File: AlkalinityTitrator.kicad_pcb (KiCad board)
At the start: 2 copper layers, 88.5 x 86.1 mm, 45 parts, among them J1 Conn_01x16, J10 Screw_Terminal_01x02, J12 V_OFFSET, J14 Conn_01x02, J2 Raspberry_Pi_2_3, J3 Conn_01x08, J4 Screw_Terminal_01x04_titrator, J5 RF_Shield_Two_Pieces, J7 SJ-43515TS, J8 Screw_Terminal_01x03, J9 SJ-43515TS, Q1 PN2222A, U1 ADS1115_BO, U2 A4988_BO, U3 MAX31865_BO, U4 MAX31865_BO, U5 LT1634, U6 LMC662, U7 LMC662, U8 L7805

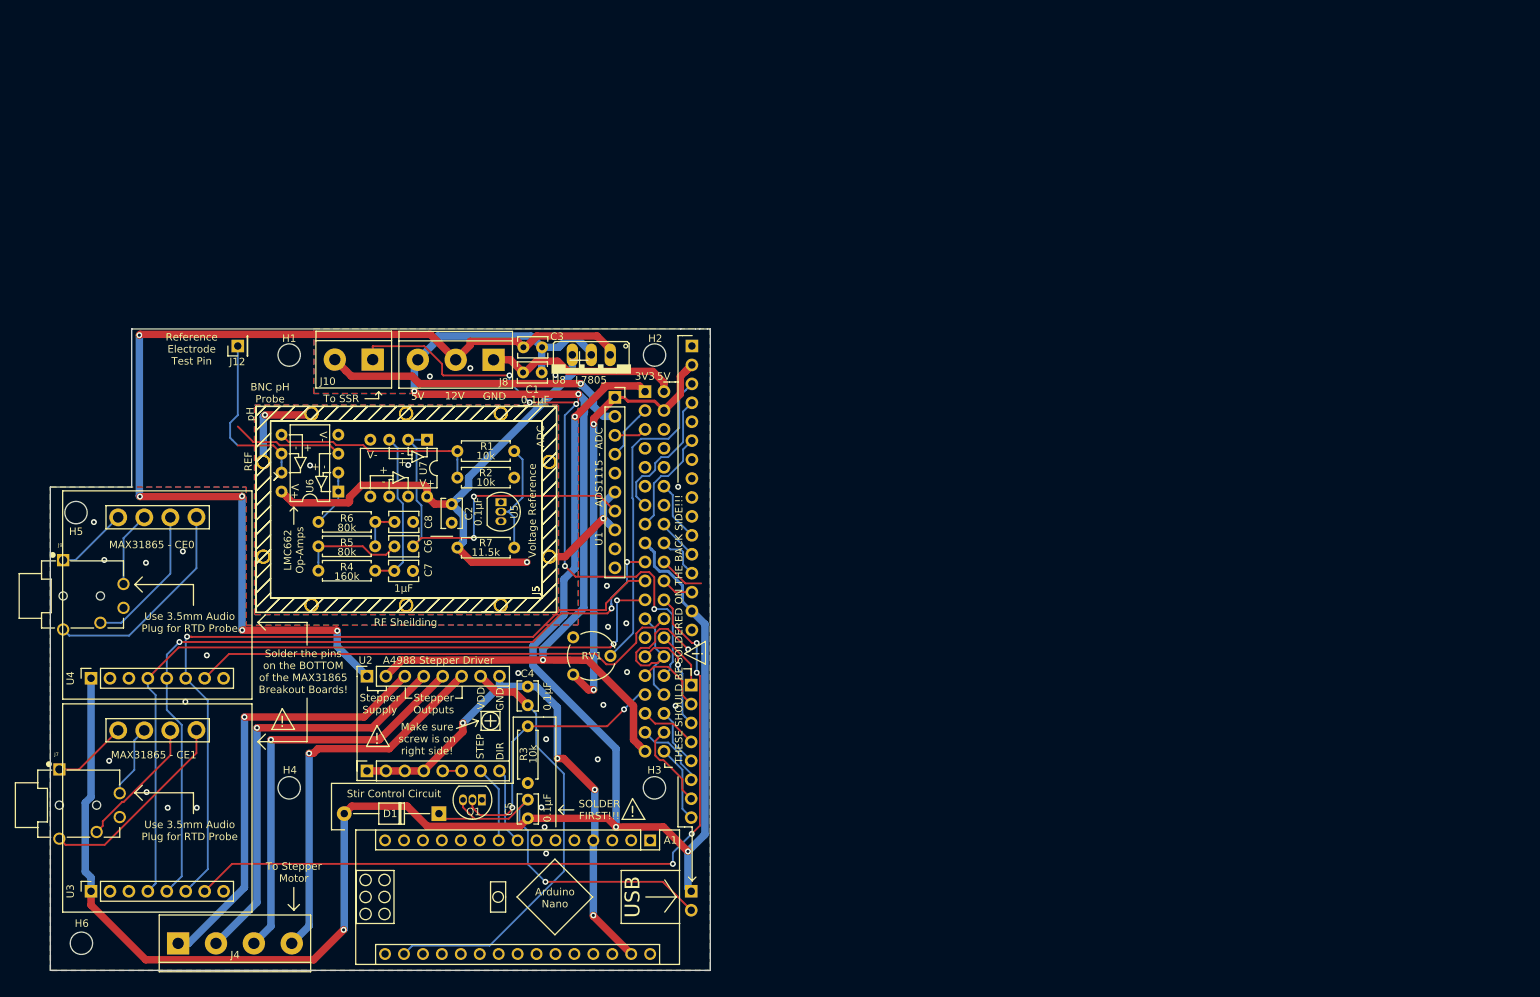
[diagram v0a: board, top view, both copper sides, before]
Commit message: rcb rev 3 start
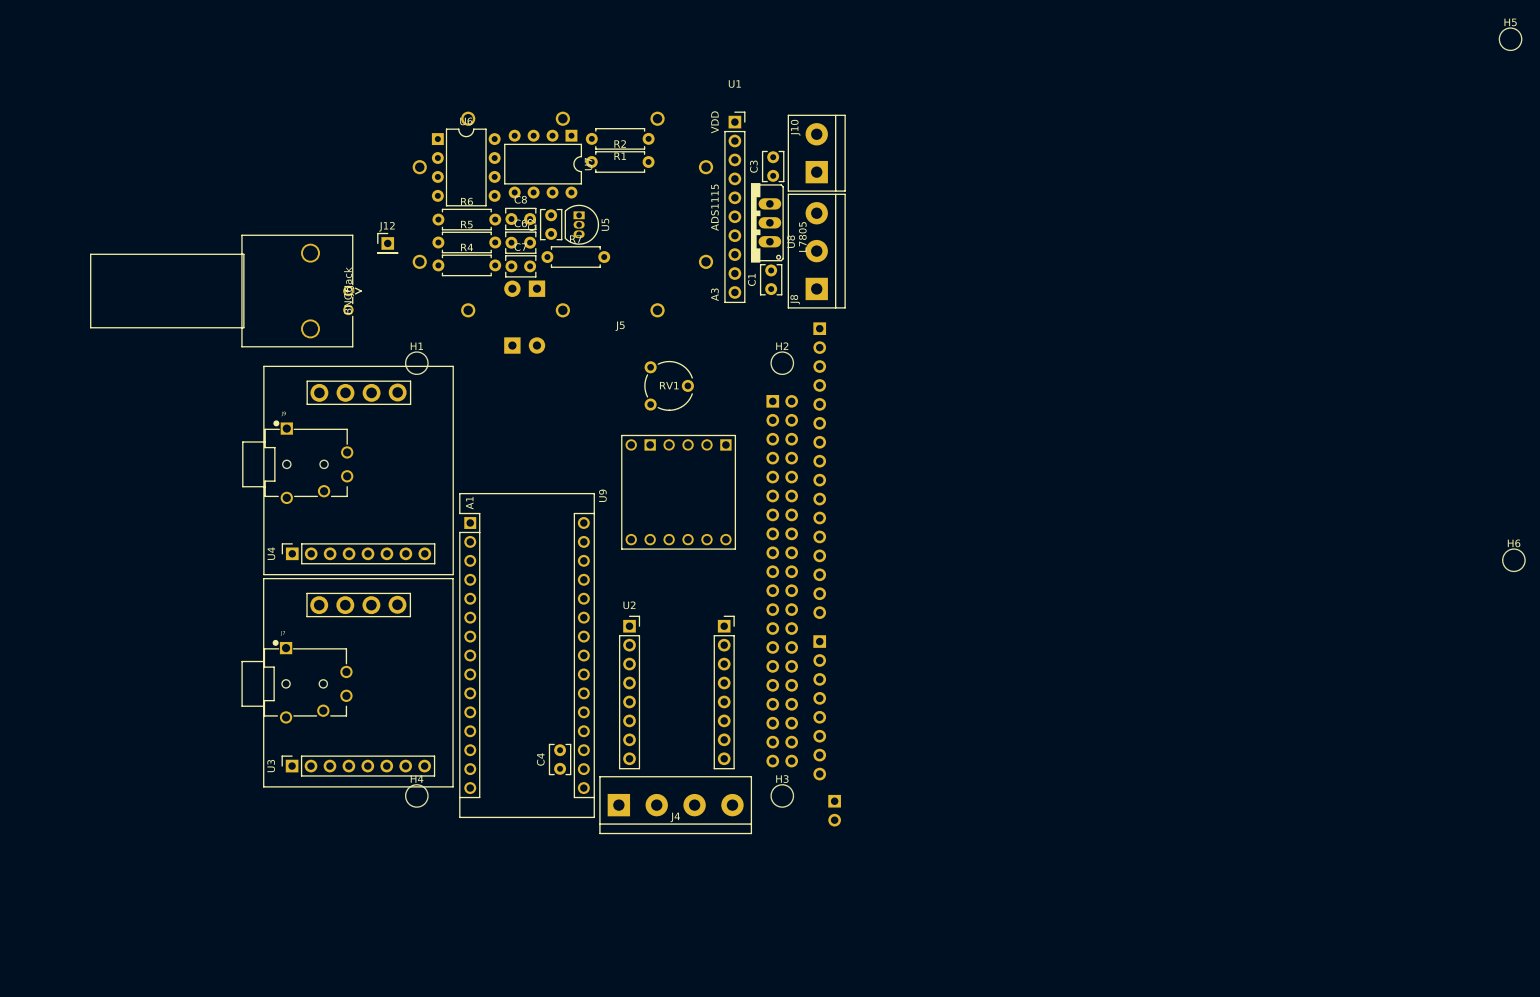
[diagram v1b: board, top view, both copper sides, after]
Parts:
- removed C5: 0.1uF, Capacitor_THT:C_Disc_D3.8mm_W2.6mm_P2.50mm
- removed the J5 at (148.2, 81.7) (x2)
- removed Q1: PN2222A, Package_TO_SOT_THT:TO-92_Inline
- removed R3: 10k, Resistor_THT:R_Axial_DIN0207_L6.3mm_D2.5mm_P7.62mm_Horizontal
- added D2: 1N5817-TP, Diode_THT:D_DO-41_SOD81_P7.62mm_Horizontal, B.Cu at (162.4, 58.9)
- added J5: RF_Shield_Two_Pieces, Titrator_Footprints:44-CBSA-1.0X1.5X0.4, F.Cu at (188.4, 54.1)
- added J6: BNC_Jack, Titrator_Footprints:BNC_Jack, F.Cu at (140.4, 51.5)
- added U9: BD65496MUV_BO, Titrator_Footprints:BD65496MUV_BO_Footprint, F.Cu at (174.8, 78.4)
- A1: footprint Module:Arduino_Nano -> Titrator_Footprints:Arduino_Nano
- D1: value DIODE -> 1N5817-TP; footprint Diode_THT:D_T-1_P12.70mm_Horizontal -> Diode_THT:D_DO-41_SOD81_P7.62mm_Horizontal; moved to B.Cu
- H1, H3, H5, H6: footprint MountingHole:MountingHole_3mm -> Titrator_Footprints:MountingHole_3mm
- J1: footprint Connector_PinSocket_2.54mm:PinSocket_1x16_P2.54mm_Horizontal -> Titrator_Footprints:PinSocket_1x16_P2.54mm_Horizontal
- J10: footprint TerminalBlock:TerminalBlock_bornier-2_P5.08mm -> Titrator_Footprints:TerminalBlock_bornier-2_P5.08mm
- J14: footprint Connector_PinSocket_2.54mm:PinSocket_1x02_P2.54mm_Vertical -> Titrator_Footprints:PinSocket_1x02_P2.54mm_Vertical
- J2: footprint Connector_PinSocket_2.54mm:PinSocket_2x20_P2.54mm_Vertical -> Titrator_Footprints:RaspberryPi
- J3: footprint Connector_PinSocket_2.54mm:PinSocket_1x08_P2.54mm_Horizontal -> Titrator_Footprints:PinSocket_1x08_P2.54mm_Horizontal
- J4: footprint TerminalBlock:TerminalBlock_bornier-4_P5.08mm -> Titrator_Footprints:TerminalBlock_bornier-4_P5.08mm
- J8: footprint TerminalBlock:TerminalBlock_bornier-3_P5.08mm -> Titrator_Footprints:TerminalBlock_bornier-3_P5.08mm
- RV1: footprint Potentiometer_THT:Potentiometer_Piher_PT-6-V_Vertical -> Titrator_Footprints:Potentiometer_Piher_PT-6-V_Vertical
- U5: value LT1634 -> LT1634_5V
- moved H5 202.7 mm to (296.4, 17.8)
- moved H6 198.9 mm to (296.8, 87.7)
- moved D1 71.6 mm to (165.7, 51.2), turned to 270 degrees
- moved J10 64.7 mm to (203.3, 35.6), turned to 90 degrees
- moved J4 62.0 mm to (176.7, 120.5)
- moved U6 49.1 mm to (152.4, 31.2), turned to 0 degrees
- moved A1 48.9 mm to (156.8, 82.7), turned to 0 degrees
- moved R2 46.0 mm to (173.1, 34.2)
- moved R1 45.6 mm to (180.7, 31.1)
- moved U7 45.2 mm to (170.4, 30.7)
- moved J8 44.4 mm to (203.3, 51.3), turned to 90 degrees
- moved R5 43.8 mm to (152.5, 45.0)
- moved C7 43.8 mm to (162.3, 48.2)
- moved C8 43.6 mm to (162.3, 41.9)
- moved C6 42.8 mm to (162.3, 45.1), turned to 0 degrees
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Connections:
- D1 pad 1: Net-(C5-Pad2) -> /PSU_AGND
- D1 pad 2: +3V3 -> GND
- J14 pad 1: +3V3 -> Net-(J14-Pad1)
- J14 pad 2: Net-(C5-Pad2) -> Net-(J14-Pad2)
- J2 pad 11: Net-(J2-Pad11) -> /MOT_DIR
- J2 pad 24: /CE0 -> Net-(J2-Pad24)
- J2 pad 26: /CE1 -> Net-(J2-Pad26)
- J2 pad 27: Net-(J2-Pad27) -> /CS0
- J2 pad 7: Net-(J2-Pad7) -> /CS1
- U1 pad 8: /PSU_AGND -> Net-(U1-Pad8)
- U3 pad 5: /MOSI -> /MISO
- U3 pad 6: /MISO -> /MOSI
- U3 pad 7: /CE0 -> /CS0
- U4 pad 5: /MOSI -> /MISO
- U4 pad 6: /MISO -> /MOSI
- U4 pad 7: /CE1 -> /CS1
- U7 pad 5: Net-(U7-Pad5) -> Net-(R1-Pad2)
- U7 pad 6: Net-(U7-Pad6) -> Net-(U1-Pad8)
- U7 pad 7: Net-(U7-Pad7) -> Net-(U1-Pad8)
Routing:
- net +3V3: track 260.7 -> 0.00 mm, vias 4 -> 0
- net /PSU_12V: track 142.3 -> 0.00 mm, vias 5 -> 0
- net /PSU_GND: track 138.8 -> 0.00 mm, vias 3 -> 0
- net /MOSI: track 105.3 -> 0.00 mm, vias 3 -> 0
- net /SCLK: track 103.7 -> 0.00 mm, vias 2 -> 0
- net /CE0: track 103.6 -> 0.00 mm, vias 4 -> 0
- net /MISO: track 102.5 -> 0.00 mm, vias 1 -> 0
- net Net-(J10-Pad1): track 84.9 -> 0.00 mm, vias 5 -> 0
- net GND: track 75.7 -> 0.00 mm, vias 28 -> 0
- net /Arduino_GND: track 71.3 -> 0.00 mm, vias 4 -> 0
- net /PSU_A5V: track 70.2 -> 0.00 mm, vias 1 -> 0
- net /CE1: track 66.8 -> 0.00 mm
- net +5V: track 60.3 -> 0.00 mm, vias 2 -> 0
- net Net-(J4-Pad1): track 58.7 -> 0.00 mm, vias 1 -> 0
- net /Arduino_VDD: track 58.3 -> 0.00 mm
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- removed copper zone on B.Cu, net /PSU_AGND
- removed copper zone on F.Cu, net /PSU_AGND
- removed copper zone on B.Cu, net GND
- removed copper zone on F.Cu, net GND
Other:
- board outline removed
- board text removed: "!"
- board text removed: "+"
- board text removed: "-"
- board text removed: "- ADC"
- board text removed: "0.1μF"
- board text removed: "10k"
- board text removed: "11.5k"
- board text removed: "12V"
- board text removed: "160k"
- board text removed: "1μF"
- board text removed: "3V3"
- board text removed: "4x4 Keypad"
- board text removed: "5V"
- board text removed: "80k"
- board text removed: "A4988 Stepper Driver"
- board text removed: "Arduino Nano"
- board text removed: "BNC pH Probe"
- board text removed: "DIR"
- board text removed: "GND"
- board text removed: "J1, J2, J3, J4 All Mounted On The Back Side!!"
- board text removed: "LCD"
- board text removed: "LMC662 Op-Amps"
- board text removed: "MAX31865 - CE0"
- board text removed: "MAX31865 - CE1"
- board text removed: "Magnetic Stirrer Motor"
- board text removed: "Make sure screw is on right side!"
- board text removed: "REF"
- board text removed: "RF Sheilding"
- board text removed: "Raspberry Pi"
- board text removed: "Reference Electrode Test Pin"
- board text removed: "SOLDER FIRST!!!"
- board text removed: "STEP"
- board text removed: "Solder the pins on the BOTTOM of the MAX31865 Breakout Boards!"
- board text removed: "Stepper Outputs"
- board text removed: "Stepper Supply"
- board text removed: "Stir Control Circuit"
- board text removed: "THESE SHOULD BE SOLDERED ON THE BACK SIDE!!!"
- board text removed: "To SSR"
- board text removed: "To Stepper Motor"
- board text removed: "USB"
- board text removed: "Use 3.5mm Audio Plug for RTD Probe"
- board text removed: "V+"
- board text removed: "V-"
- board text removed: "VDD"
- board text removed: "Voltage Reference"
- board text removed: "WWU Alkalinity Titrator Rev. 2.0 Made By: Konrad McClure and Noah Griffith 2021 Team"
- board text removed: "pH"

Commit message: sleep is for losers. Did layout for Rev 3 board
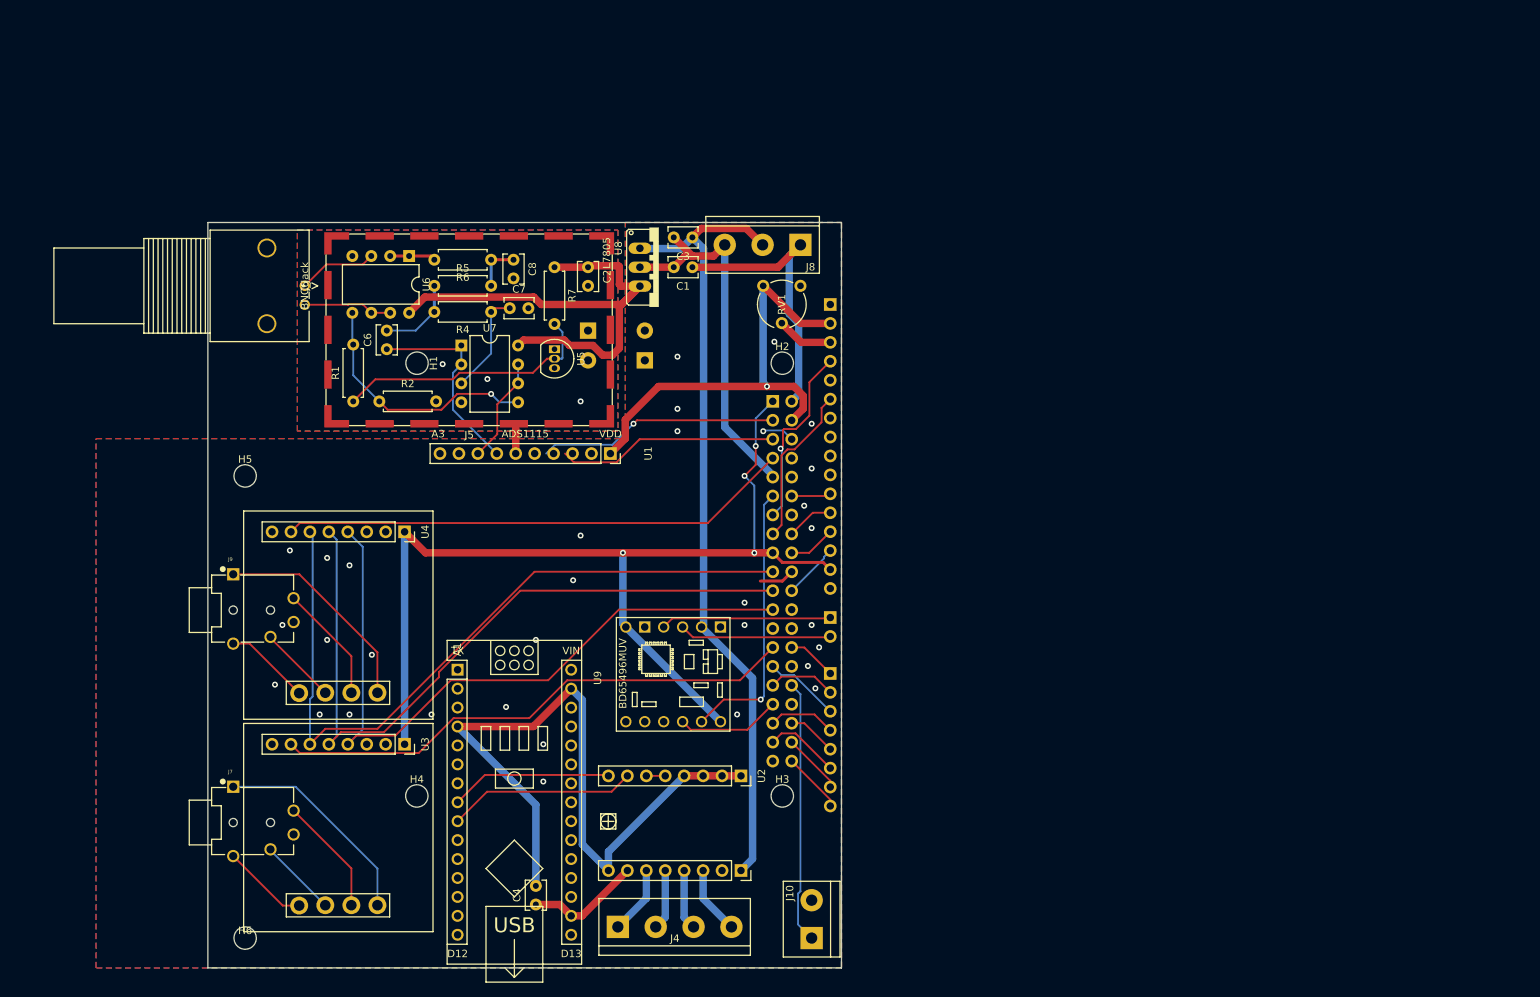
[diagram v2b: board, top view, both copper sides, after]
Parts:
- removed J12: V_OFFSET, Connector_PinHeader_2.54mm:PinHeader_1x01_P2.54mm_Vertical
- J1: footprint Titrator_Footprints:PinSocket_1x16_P2.54mm_Horizontal -> Titrator_Footprints:PinHeader_1x16_P2.54mm_Horizontal
- J14: footprint Titrator_Footprints:PinSocket_1x02_P2.54mm_Vertical -> Titrator_Footprints:PinHeader_1x02_P2.54mm_Horizontal
- J3: footprint Titrator_Footprints:PinSocket_1x08_P2.54mm_Horizontal -> Titrator_Footprints:PinHeader_1x08_P2.54mm_Horizontal
- J5: footprint Titrator_Footprints:44-CBSA-1.0X1.5X0.4 -> Titrator_Footprints:SMS-205_LeaderTech_RFShield
- moved H5 179.6 mm to (126.6, 76.4)
- moved H6 177.6 mm to (126.6, 138.4)
- moved J10 102.8 mm to (202.6, 138.4)
- moved R1 53.0 mm to (141.1, 66.4), turned to 90 degrees
- moved U1 47.5 mm to (175.6, 73.4), turned to 270 degrees
- moved R2 42.9 mm to (144.6, 66.4)
- moved U7 31.8 mm to (155.6, 58.9), turned to 0 degrees
- moved U2 25.7 mm to (193.6, 116.4), turned to 270 degrees
- moved J14 24.7 mm to (205.1, 95.4)
- moved U9 24.4 mm to (174.1, 102.9)
- moved C6 22.0 mm to (145.6, 59.4), turned to 90 degrees
- moved RV1 21.9 mm to (196.1, 50.9), turned to 270 degrees
- moved J9 20.8 mm to (127.6, 94.4)
- moved J5 20.0 mm to (176.1, 69.9)
- moved J7 19.9 mm to (127.6, 122.9)
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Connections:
- J2 pad 39: /PSU_GND -> GND
- J2 pad 9: GND -> /PSU_GND
- U2 pad 10: /PSU_GND -> GND
- U2 pad 11: Net-(J4-Pad1) -> Net-(J4-Pad4)
- U2 pad 12: Net-(J4-Pad2) -> Net-(J4-Pad3)
- U2 pad 13: Net-(J4-Pad3) -> Net-(J4-Pad2)
- U2 pad 14: Net-(J4-Pad4) -> Net-(J4-Pad1)
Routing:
- net +3V3: track 0.00 -> 138.2 mm, vias 0 -> 4
- net /PSU_12V: track 0.00 -> 107.7 mm
- net /MOSI: track 0.00 -> 100.5 mm
- net /MISO: track 0.00 -> 97.9 mm
- net /SCLK: track 0.00 -> 94.7 mm
- net /Arduino_GND: track 0.00 -> 94.1 mm
- net /PSU_A5V: track 0.00 -> 72.7 mm
- net /CS0: track 0.00 -> 71.0 mm
- net /CS1: track 0.00 -> 68.7 mm
- net +5V: track 0.00 -> 60.3 mm, vias 0 -> 1
- net /PSU_GND: track 0.00 -> 50.0 mm
- net /PSU_5V: track 0.00 -> 38.3 mm
- net /MOT_DIR: track 0.00 -> 37.1 mm, vias 0 -> 1
- net Net-(R1-Pad1): track 0.00 -> 35.5 mm
- net Net-(J10-Pad1): track 0.00 -> 35.3 mm
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- added copper zone on B.Cu, net /PSU_AGND
- added copper zone on F.Cu, net /PSU_AGND
- added copper zone on B.Cu, net GND
- added copper zone on F.Cu, net GND
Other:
- board outline added: 85 x 100 mm
